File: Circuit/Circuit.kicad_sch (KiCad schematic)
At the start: 16 parts, among them J1 Conn_01x20, J2 Conn_01x20, U1 TL072, U2 AMS1117-3.3, Y1 Crystal

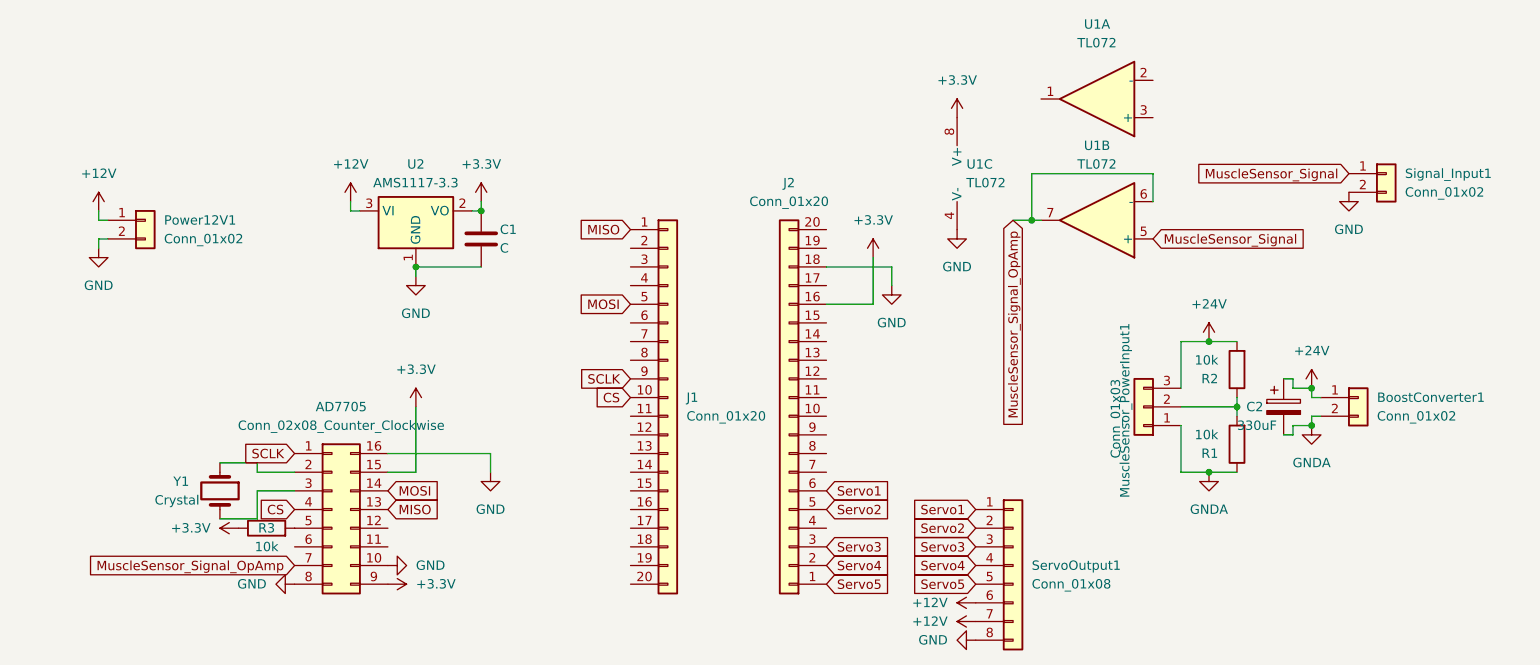
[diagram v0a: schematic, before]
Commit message: final PCB design done
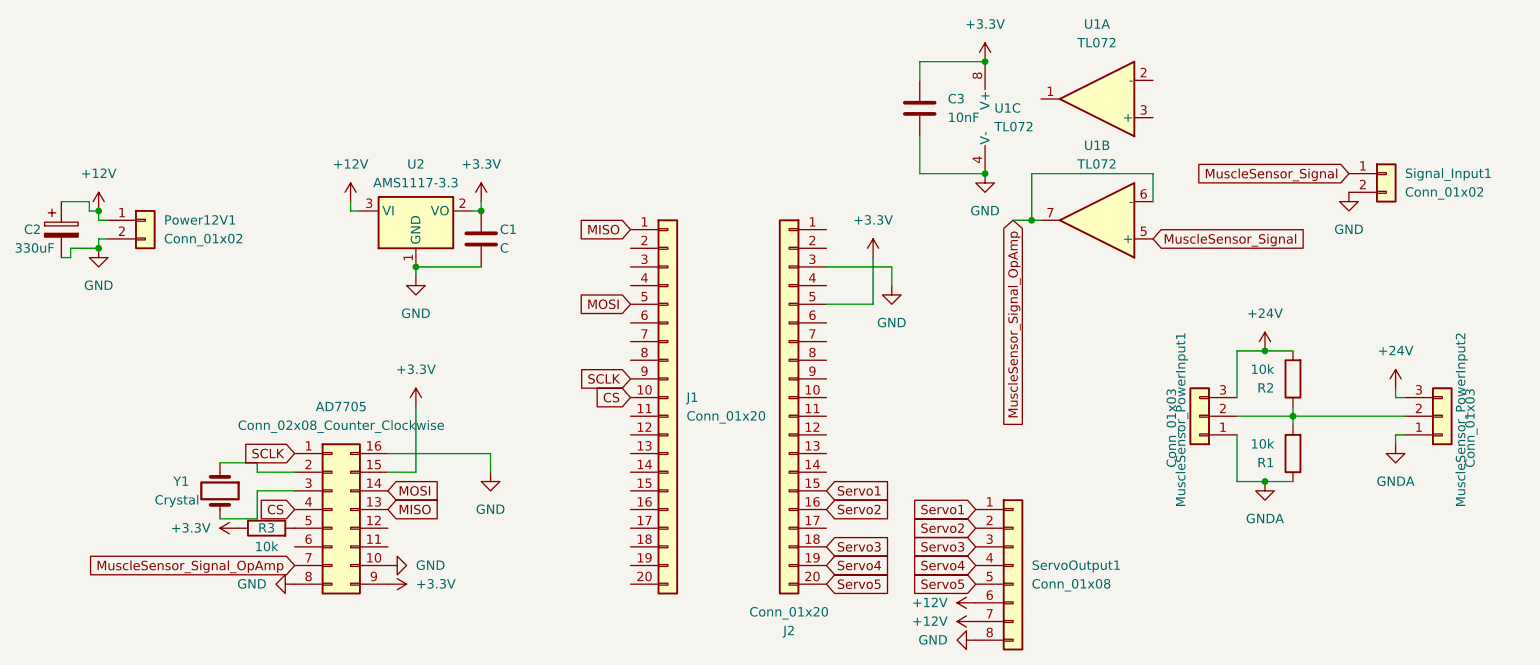
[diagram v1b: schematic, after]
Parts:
- removed BoostConverter1: Conn_01x02, Connector_JST:JST_EH_B2B-EH-A_1x02_P2.50mm_Vertical, symbol Connector_Generic:Conn_01x02
- added C3: 10nF, Capacitor_THT:C_Disc_D5.0mm_W2.5mm_P5.00mm, symbol Device:C
- added MuscleSensor_PowerInput2: Conn_01x03, Connector_JST:JST_EH_S3B-EH_1x03_P2.50mm_Horizontal, symbol Connector_Generic:Conn_01x03
- C2: footprint (none) -> Capacitor_THT:CP_Radial_D8.0mm_P3.80mm
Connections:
- net +12V: now also C2.1
- net +24V: now also MuscleSensor_PowerInput2.3 (Pin_3); no longer C2.1
- net +3.3V: now also J2.5 (Pin_5), C3.1; no longer J2.16 (Pin_16)
- net GND: now also C2.2, J2.3 (Pin_3), C3.2; no longer J2.18 (Pin_18)
- net GNDA: now also MuscleSensor_PowerInput2.1 (Pin_1); no longer C2.2
- net Servo1: now also J2.15 (Pin_15); no longer J2.6 (Pin_6)
- net Servo2: now also J2.16 (Pin_16); no longer J2.5 (Pin_5)
- net Servo3: now also J2.18 (Pin_18); no longer J2.3 (Pin_3)
- net Servo4: now also J2.19 (Pin_19); no longer J2.2 (Pin_2)
- net Servo5: now also J2.20 (Pin_20); no longer J2.1 (Pin_1)
- net at MuscleSensor_PowerInput1.2 (Pin_2), R1.2, R2.1: now also MuscleSensor_PowerInput2.2 (Pin_2)
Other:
- moved on the sheet: C2, J2, MuscleSensor_PowerInput1, R1, R2, U1C
